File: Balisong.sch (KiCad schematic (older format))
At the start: 24 parts, among them J1 USB_B_Micro, SW1 SW_Push, U1 ATmega32U4-AU, Y1 16MHz

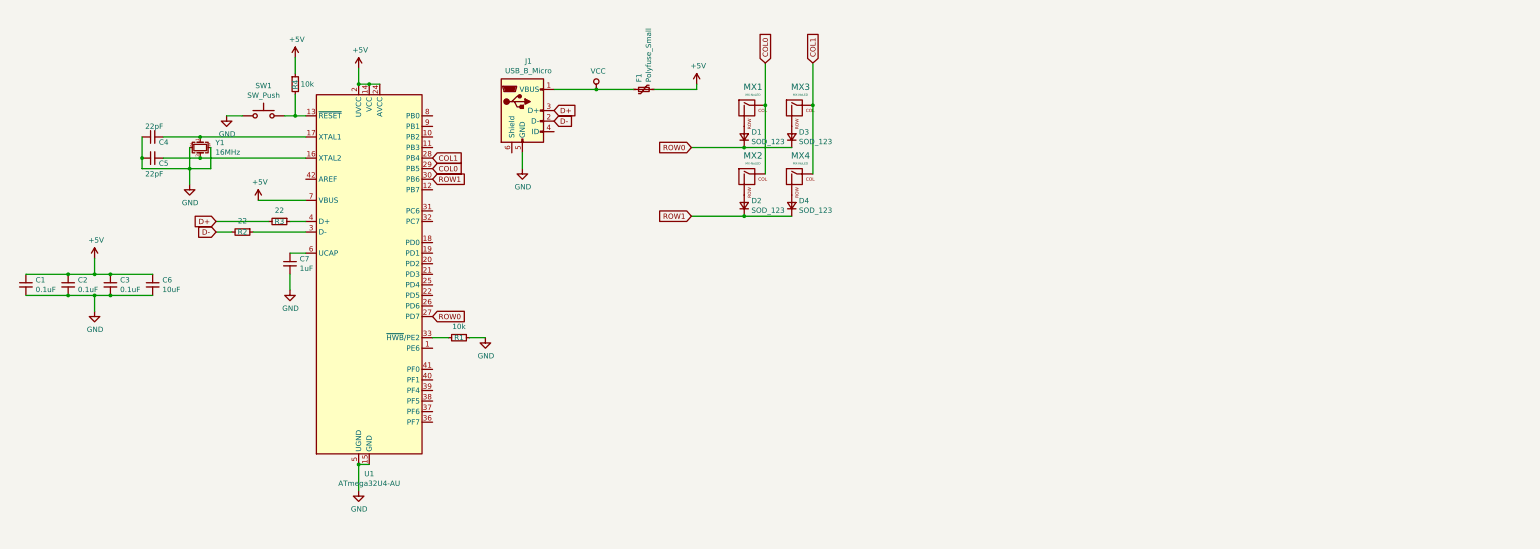
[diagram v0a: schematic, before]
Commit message: Update
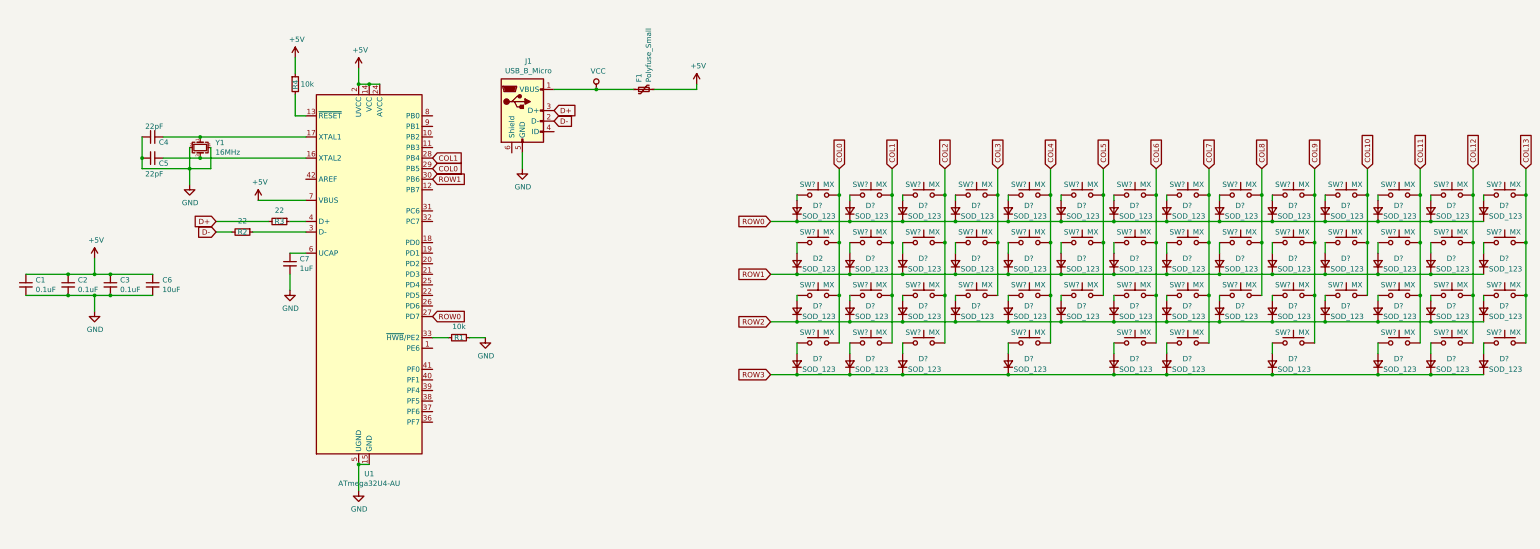
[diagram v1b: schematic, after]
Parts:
- removed D1, D3, D4: SOD_123, Diode_SMD:D_SOD-123, symbol Device:D_Small
- removed MX1, MX2, MX3, MX4: MX-NoLED, MX_Alps_Hybrid:MX-1U, symbol MX_Alps_Hybrid:MX-NoLED
- removed SW1: SW_Push, random-keyboard-parts:SKQG-1155865, symbol Switch:SW_Push
- added D? (x51): SOD_123, Diode_SMD:D_SOD-123, symbol Device:D_Small
- added SW? (x52): MX, symbol Switch:SW_Push
- F1: footprint Fuse:Fuse_1206_3216Metric_Pad1.42x1.75mm_HandSolder -> Fuse:Fuse_1206_3216Metric_Castellated
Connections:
- net COL0: now also SW?.2, SW?.2, SW?.2, SW?.2
- net COL1: now also SW?.2, SW?.2, SW?.2, SW?.2
- net ROW0: now also D?.1 (K), D?.1 (K), D?.1 (K), D?.1 (K), D?.1 (K), D?.1 (K), D?.1 (K), D?.1 (K), D?.1 (K), D?.1 (K), D?.1 (K), D?.1 (K), D?.1 (K), D?.1 (K)
- net ROW1: now also D?.1 (K), D?.1 (K), D?.1 (K), D?.1 (K), D?.1 (K), D?.1 (K), D?.1 (K), D?.1 (K), D?.1 (K), D?.1 (K), D?.1 (K), D?.1 (K), D?.1 (K)
- net at D2.2 (A): now also SW?.1
- new net: D?.2 (A), SW?.1 (x51)
- new net COL10: SW?.2, SW?.2, SW?.2
- new net COL11: SW?.2, SW?.2, SW?.2, SW?.2
- new net COL12: SW?.2, SW?.2, SW?.2, SW?.2
- new net COL13: SW?.2, SW?.2, SW?.2, SW?.2
- new net COL2: SW?.2, SW?.2, SW?.2, SW?.2
- new net COL3: SW?.2, SW?.2, SW?.2
- new net COL4: SW?.2, SW?.2, SW?.2, SW?.2
- new net COL5: SW?.2, SW?.2, SW?.2
- new net COL6: SW?.2, SW?.2, SW?.2, SW?.2
- new net COL7: SW?.2, SW?.2, SW?.2, SW?.2
- new net COL8: SW?.2, SW?.2, SW?.2
- new net COL9: SW?.2, SW?.2, SW?.2, SW?.2
- new net ROW2: D?.1 (K), D?.1 (K), D?.1 (K), D?.1 (K), D?.1 (K), D?.1 (K), D?.1 (K), D?.1 (K), D?.1 (K), D?.1 (K), D?.1 (K), D?.1 (K), D?.1 (K), D?.1 (K)
- new net ROW3: D?.1 (K), D?.1 (K), D?.1 (K), D?.1 (K), D?.1 (K), D?.1 (K), D?.1 (K), D?.1 (K), D?.1 (K), D?.1 (K)
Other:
- moved on the sheet: D2

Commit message: Finished pcb
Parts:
- removed C3: 0.1uF, Capacitor_SMD:C_0805_2012Metric, symbol Device:C_Small
- removed F1: Polyfuse_Small, Fuse:Fuse_1206_3216Metric_Castellated, symbol Device:Polyfuse_Small
- removed Y1: 16MHz, Crystal:Crystal_SMD_3225-4Pin_3.2x2.5mm, symbol Device:Crystal_GND24_Small
- added C1: 0.1uF, Capacitor_SMD:C_0805_2012Metric_Pad1.15x1.40mm_HandSolder, symbol Device:C_Small
- added SW53: SW_Push, Button_Switch_SMD:SW_SPST_B3U-1000P, symbol Switch:SW_Push
- added Y1: 16MHz, Crystal:Crystal_SMD_Abracon_ABM3-2Pin_5.0x3.2mm_HandSoldering, symbol Device:Crystal_Small
- C2: renamed from C1; footprint Capacitor_SMD:C_0805_2012Metric -> Capacitor_SMD:C_0805_2012Metric_Pad1.15x1.40mm_HandSolder
- C3: renamed from C2; footprint Capacitor_SMD:C_0805_2012Metric -> Capacitor_SMD:C_0805_2012Metric_Pad1.15x1.40mm_HandSolder
- C5: renamed from C7; footprint Capacitor_SMD:C_0805_2012Metric -> Capacitor_SMD:C_0805_2012Metric_Pad1.15x1.40mm_HandSolder
- C6: footprint Capacitor_SMD:C_0805_2012Metric -> Capacitor_SMD:C_0805_2012Metric_Pad1.15x1.40mm_HandSolder
- C7: renamed from C4; footprint Capacitor_SMD:C_0805_2012Metric -> Capacitor_SMD:C_0805_2012Metric_Pad1.15x1.40mm_HandSolder
- C8: renamed from C5; footprint Capacitor_SMD:C_0805_2012Metric -> Capacitor_SMD:C_0805_2012Metric_Pad1.15x1.40mm_HandSolder
- R1, R3: footprint Resistor_SMD:R_0805_2012Metric -> Resistor_SMD:R_0805_2012Metric_Pad1.15x1.40mm_HandSolder
- R2: renamed from R4; footprint Resistor_SMD:R_0805_2012Metric -> Resistor_SMD:R_0805_2012Metric_Pad1.15x1.40mm_HandSolder
- R4: renamed from R2; footprint Resistor_SMD:R_0805_2012Metric -> Resistor_SMD:R_0805_2012Metric_Pad1.15x1.40mm_HandSolder
- SW1, SW25, SW29, SW49: renamed from SW?; footprint (none) -> Button_Switch_Keyboard:SW_Cherry_MX_1.50u_PCB
- SW10, SW11, SW13, SW14, SW15, SW16, SW17, SW18, SW20, SW21, SW22, SW23, SW26, SW27, SW3, SW30, SW31, SW32, SW33, SW34, SW35, SW36, SW38, SW39, SW40, SW41, SW42, SW43, SW45, SW46, SW47, SW5, SW51, SW6, SW7, SW9: renamed from SW?; footprint (none) -> Button_Switch_Keyboard:SW_Cherry_MX_1.00u_PCB
- SW12, SW2, SW24, SW28, SW4, SW44, SW48, SW50, SW52, SW8: renamed from SW?; footprint (none) -> Button_Switch_Keyboard:SW_Cherry_MX_1.25u_PCB
- SW19, SW37: renamed from SW?; footprint (none) -> Button_Switch_Keyboard:SW_Cherry_MX_2.75u_PCB
- gave numbers to parts that had none: 51
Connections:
- net labels removed: +5V
- wire segments 199 -> 193
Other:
- moved on the sheet: C2, C3, C6, J1, R3, R4
